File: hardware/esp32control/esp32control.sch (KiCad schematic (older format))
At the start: 52 parts, among them J1 Conn_02x10_Odd_Even, Q5 BSS138, Q6 BSS138, Q7 MMBT3904, Q8 MMBT3904, SW1 Boot, SW2 Reset, U1 ESP32-WROOM, U10 LTV-354T, U11 HUT4, U12 LM1117-3.3, U4 LM2675M-5, U5 LTV-354T, U8 LTV-354T, U9 LTV-354T

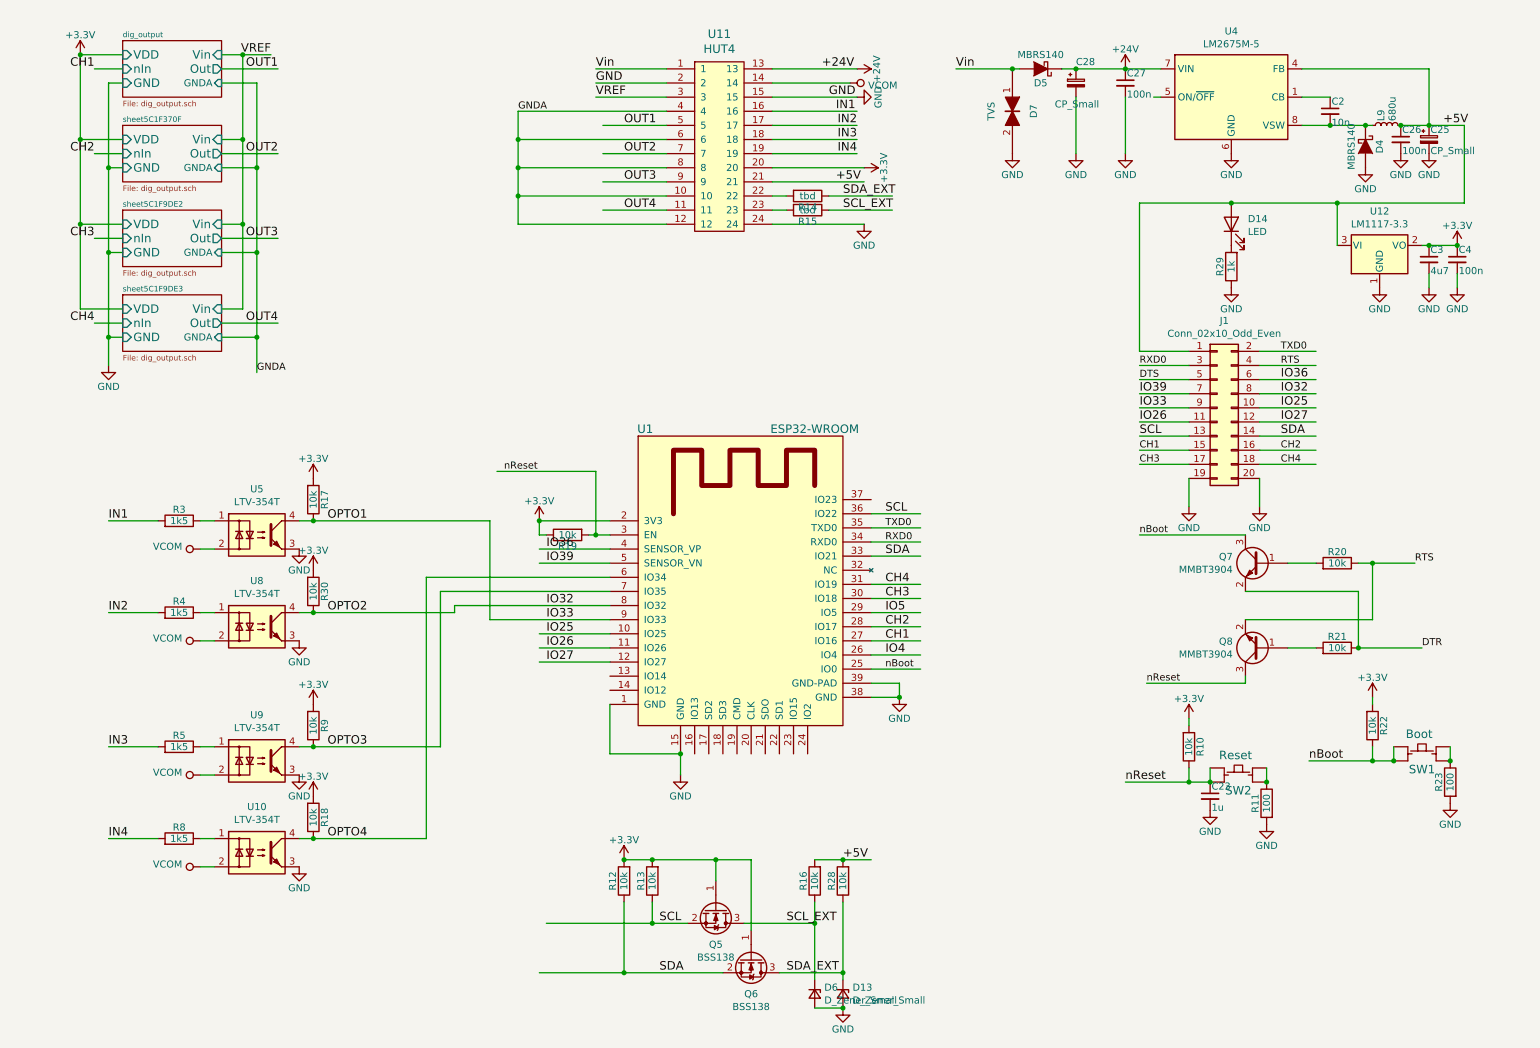
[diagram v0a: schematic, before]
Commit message: revB initial
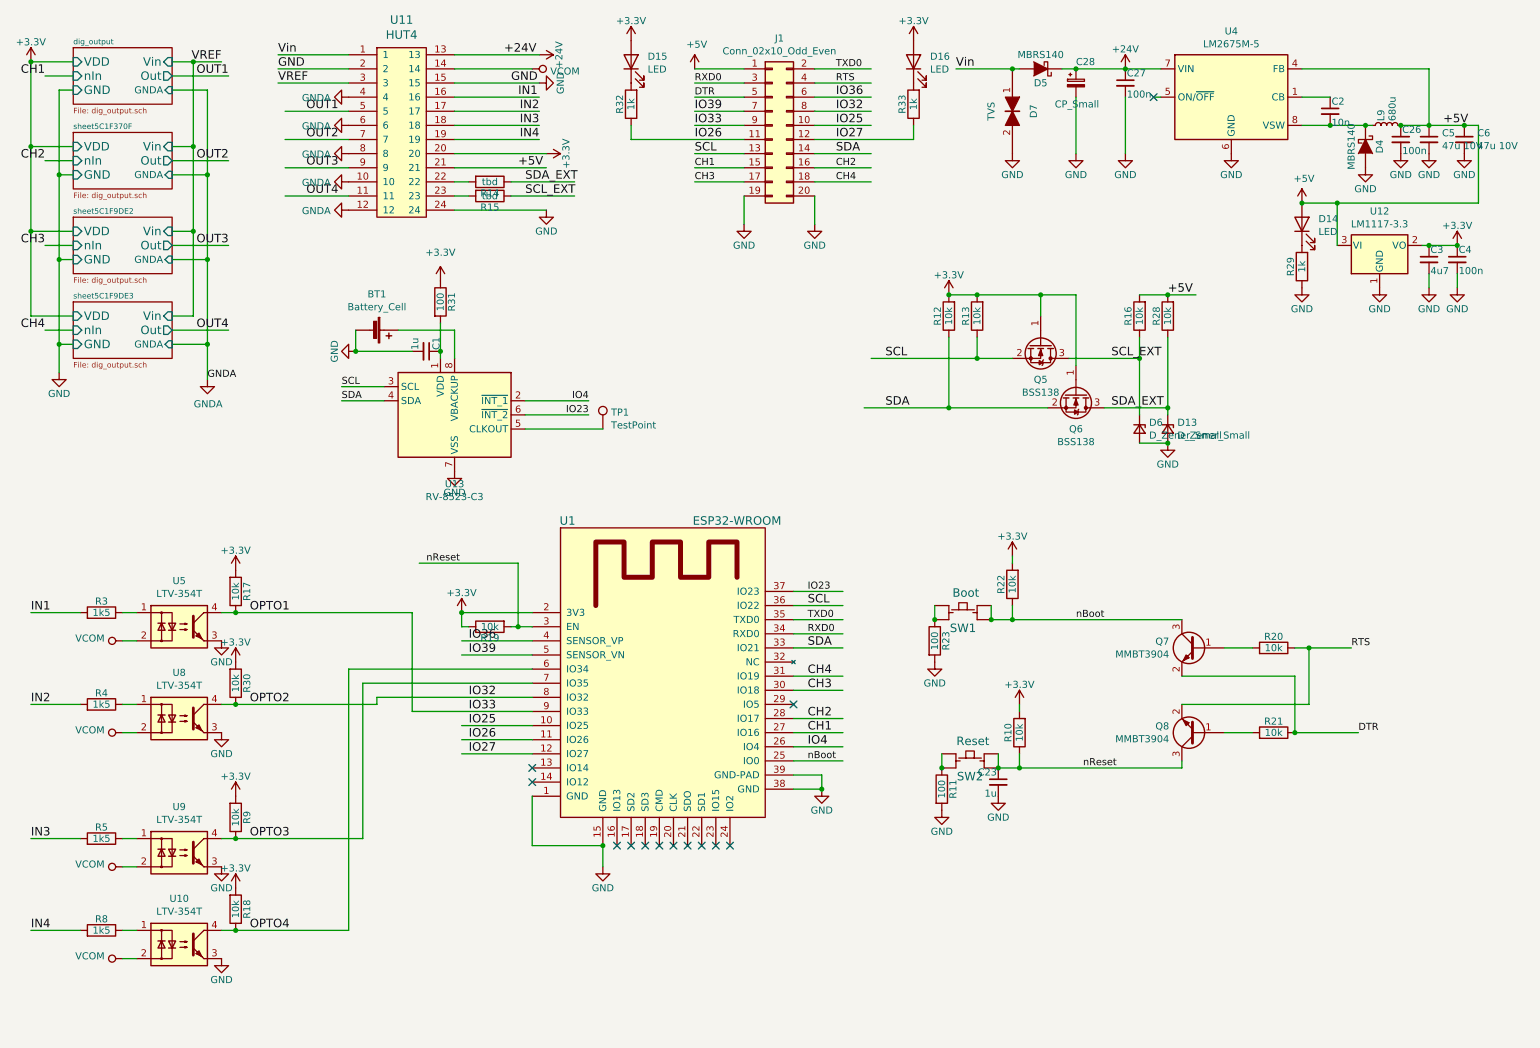
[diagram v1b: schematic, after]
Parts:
- removed C25: CP_Small, Capacitor_THT:CP_Radial_D8.0mm_P3.50mm, symbol esp32control-rescue:CP_Small-device-esp32ValveControl-rescue
- added BT1: Battery_Cell, Battery:BatteryHolder_Keystone_3001_1x12mm, symbol Device:Battery_Cell
- added C1: 1u, Capacitor_SMD:C_0603_1608Metric, symbol esp32control-rescue:C_Small-device-esp32ValveControl-rescue
- added C5, C6: 47u 10V, Capacitor_SMD:C_1206_3216Metric, symbol Device:C_Small
- added D15, D16: LED, LED_SMD:LED_0603_1608Metric_Pad1.05x0.95mm_HandSolder, symbol Device:LED
- added R31: 100, Resistor_SMD:R_0603_1608Metric, symbol Device:R
- added R32, R33: 1k, Resistor_SMD:R_0603_1608Metric, symbol Device:R
- added TP1: TestPoint, TestPoint:TestPoint_Pad_D1.5mm, symbol Connector:TestPoint
- added U13: RV-8523-C3, Package_SON:RTC_SMD_MicroCrystal_C3_2.5x3.7mm, symbol Timer_RTC:RV-8523-C3
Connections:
- net labels added: IO23
- net labels removed: DTS, IO5
- wire segments 216 -> 217
- no-connect marks 0 -> 13
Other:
- moved on the sheet: C23, D13, D14, D6, J1, Q5, Q6, Q7, Q8, R10, R11, R12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
